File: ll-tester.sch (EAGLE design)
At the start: 133 parts, among them IC1 BMA490L, IC2 TCAN330GD, IC3 EM14R0D-R20-L064S, IC4 CAT4238TD-GT3, U1 PIC32MK0512MCJ048T-I/Y8XTQFP4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, U2 MAX6126B30, U3 BNO080, U4 BME280, U5 VCNL4040M3OE

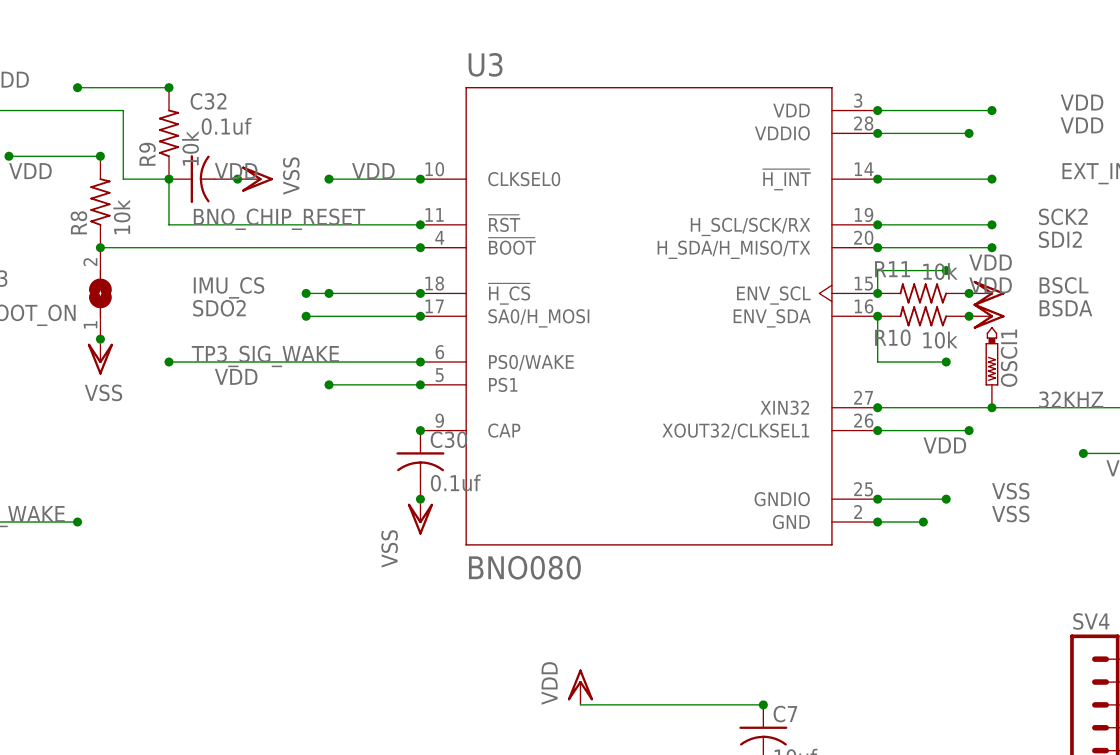
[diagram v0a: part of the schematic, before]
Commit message: up
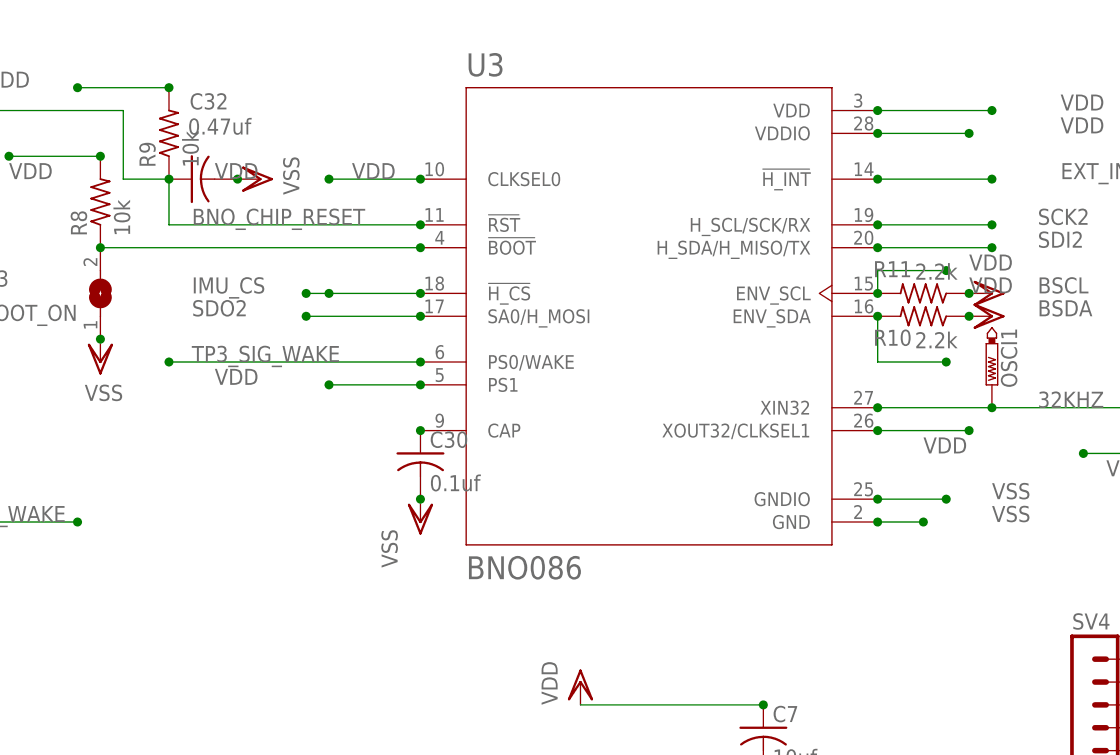
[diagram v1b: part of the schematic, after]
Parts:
- C32: value 0.1uf -> 0.47uf
- R10, R11: value 10k -> 2.2k
- U3: value BNO080 -> BNO086
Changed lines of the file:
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@@
 <part name="R7" library="rcl" library_urn="urn:adsk.eagle:library:334" deviceset="R-US_" device="M0805" package3d_urn="urn:adsk.eagle:package:23556/2" value="10k"/>
 <part name="VDD18" library="supply1" library_urn="urn:adsk.eagle:library:371" deviceset="VDD" device=""/>
-<part name="U3" library="BNO080" deviceset="BNO080" device=""/>
+<part name="U3" library="BNO080" deviceset="BNO080" device="" value="BNO086"/>
 <part name="C30" library="rcl" library_urn="urn:adsk.eagle:library:334" deviceset="C-US" device="C0805" package3d_urn="urn:adsk.eagle:package:23617/2" value="0.1uf"/>
 <part name="VSS60" library="supply1" library_urn="urn:adsk.eagle:library:371" deviceset="VSS" device=""/>
@@
 <part name="SJ3" library="jumper" library_urn="urn:adsk.eagle:library:252" deviceset="SJ" device="" package3d_urn="urn:adsk.eagle:package:15471/1" value="BOOT_ON"/>
 <part name="R9" library="rcl" library_urn="urn:adsk.eagle:library:334" deviceset="R-US_" device="M0805" package3d_urn="urn:adsk.eagle:package:23556/2" value="10k"/>
-<part name="C32" library="rcl" library_urn="urn:adsk.eagle:library:334" deviceset="C-US" device="C0805" package3d_urn="urn:adsk.eagle:package:23617/2" value="0.1uf"/>
+<part name="C32" library="rcl" library_urn="urn:adsk.eagle:library:334" deviceset="C-US" device="C0805" package3d_urn="urn:adsk.eagle:package:23617/2" value="0.47uf"/>
 <part name="VSS62" library="supply1" library_urn="urn:adsk.eagle:library:371" deviceset="VSS" device=""/>
 <part name="SJ4" library="jumper" library_urn="urn:adsk.eagle:library:252" deviceset="SJ" device="" package3d_urn="urn:adsk.eagle:package:15471/1" value="IMU_RESET"/>
@@
 <part name="SV4" library="con-lstb" library_urn="urn:adsk.eagle:library:162" deviceset="MA10-1" device="" package3d_urn="urn:adsk.eagle:package:8346/1" value="IMU_SIG"/>
 <part name="VSS64" library="supply1" library_urn="urn:adsk.eagle:library:371" deviceset="VSS" device=""/>
-<part name="R10" library="rcl" library_urn="urn:adsk.eagle:library:334" deviceset="R-US_" device="M0805" package3d_urn="urn:adsk.eagle:package:23556/2" value="10k"/>
-<part name="R11" library="rcl" library_urn="urn:adsk.eagle:library:334" deviceset="R-US_" device="M0805" package3d_urn="urn:adsk.eagle:package:23556/2" value="10k"/>
+<part name="R10" library="rcl" library_urn="urn:adsk.eagle:library:334" deviceset="R-US_" device="M0805" package3d_urn="urn:adsk.eagle:package:23556/2" value="2.2k"/>
+<part name="R11" library="rcl" library_urn="urn:adsk.eagle:library:334" deviceset="R-US_" device="M0805" package3d_urn="urn:adsk.eagle:package:23556/2" value="2.2k"/>
 <part name="VDD19" library="supply1" library_urn="urn:adsk.eagle:library:371" deviceset="VDD" device=""/>
 <part name="VDD24" library="supply1" library_urn="urn:adsk.eagle:library:371" deviceset="VDD" device=""/>
